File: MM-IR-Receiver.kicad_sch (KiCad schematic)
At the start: 8 parts

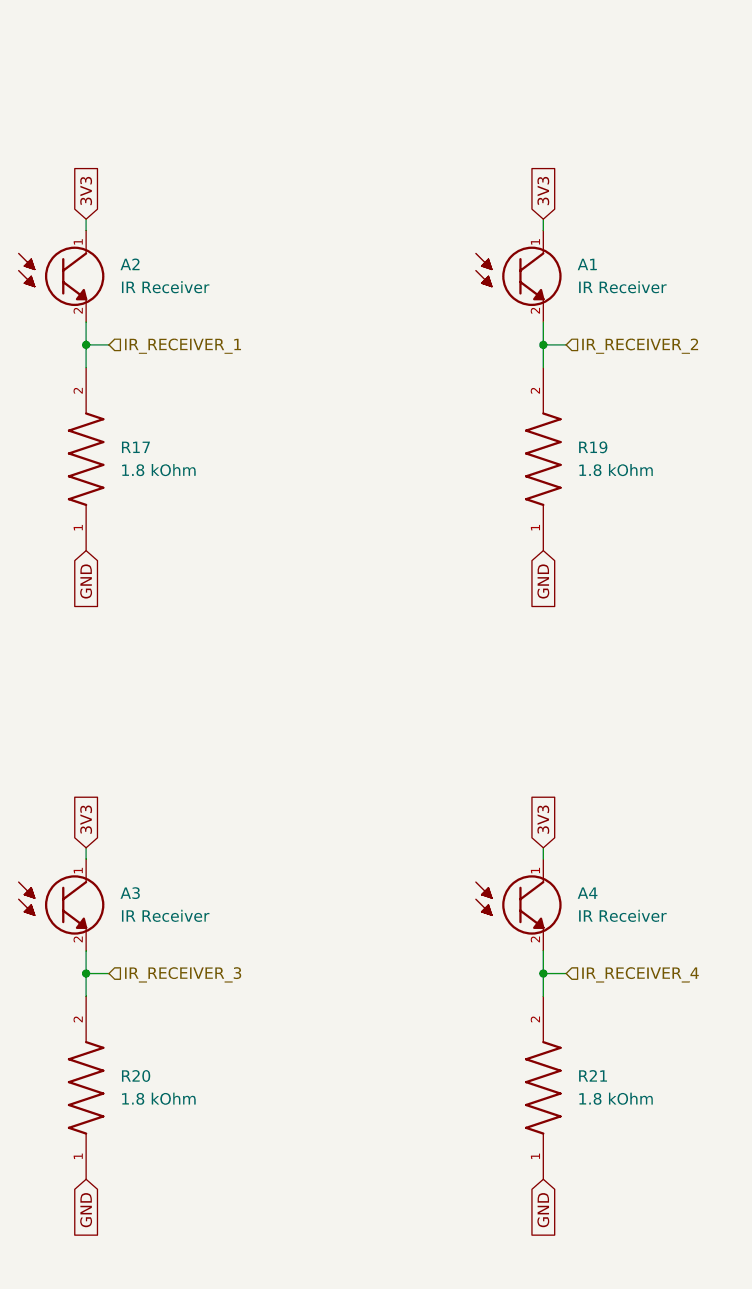
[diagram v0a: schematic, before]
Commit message: PCB tentative finished
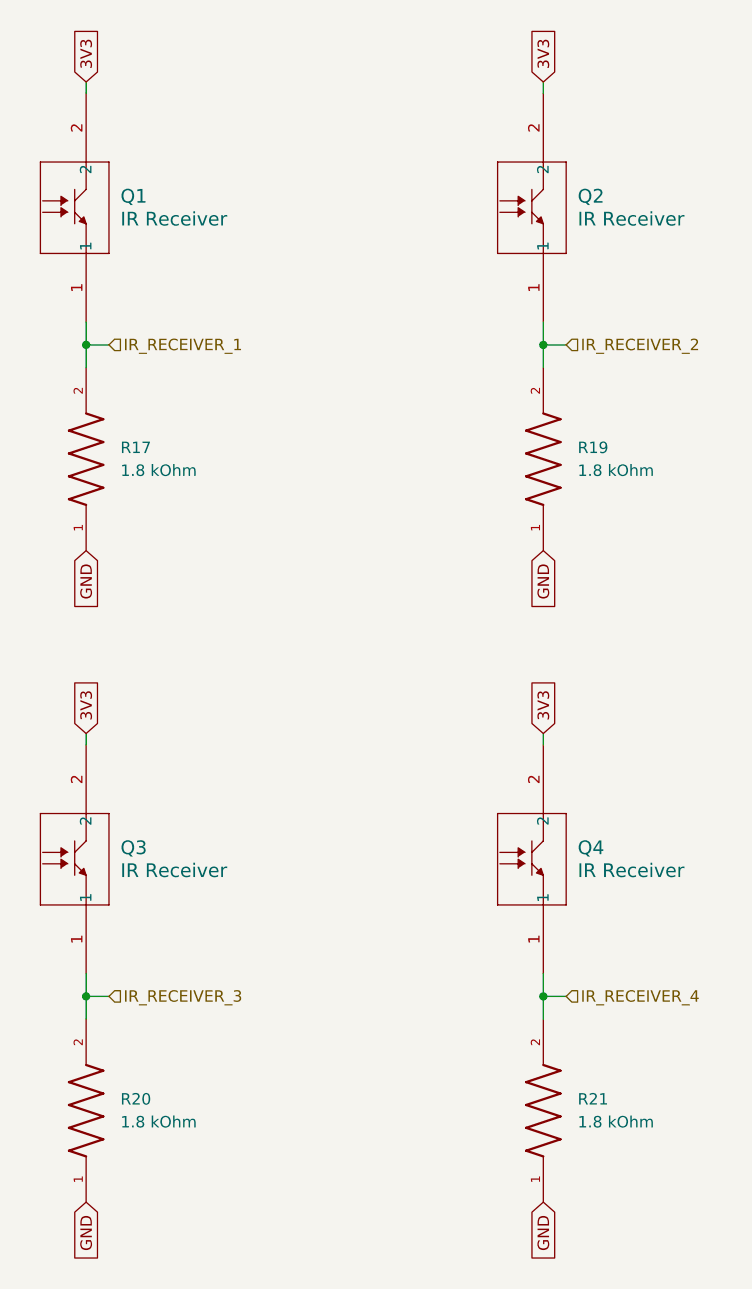
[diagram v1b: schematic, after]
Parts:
- removed A1, A2, A3, A4: IR Receiver, IR_Receiver_ALS-PT19-315C_L177_TR8:XDCR_ALS-PT19-315C_L177_TR8, symbol Phototransistor_ALS-PT19-315C_L177_TR8:ALS-PT19-315C_L177_TR8
- added Q1, Q2, Q3, Q4: IR Receiver, IR_Receiver_ul_LTR-4206E:NoneP157X157-2_LTO, symbol IR_Receiver_ul_LTR-4206E:LTR-4206E
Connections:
- net 3V3: now also Q1.2, Q2.2, Q3.2, Q4.2
- net IR_RECEIVER_1: now also Q1.1
- net IR_RECEIVER_2: now also Q2.1
- net IR_RECEIVER_3: now also Q3.1
- net IR_RECEIVER_4: now also Q4.1
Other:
- moved on the sheet: R20, R21
